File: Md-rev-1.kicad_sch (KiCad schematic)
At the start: 24 parts, among them CN1 JSTPH, J1 USB_C_Receptacle_USB2.0, J2 AudioJack4_SwitchTR1, U1 MCP73831-2-OT, U2 MAX9814

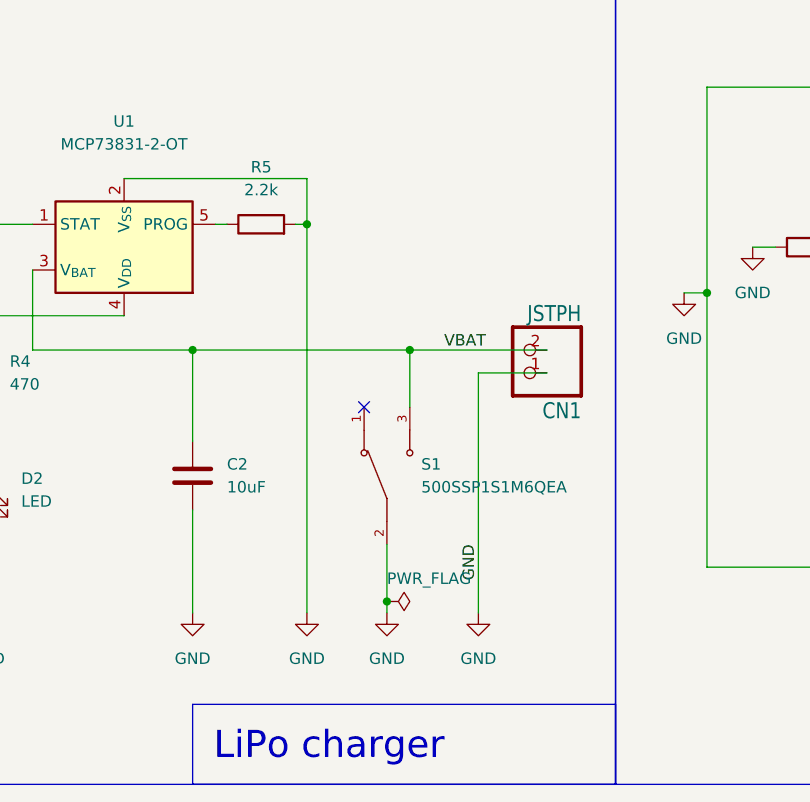
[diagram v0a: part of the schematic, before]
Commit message: Updated the schematic & PCB
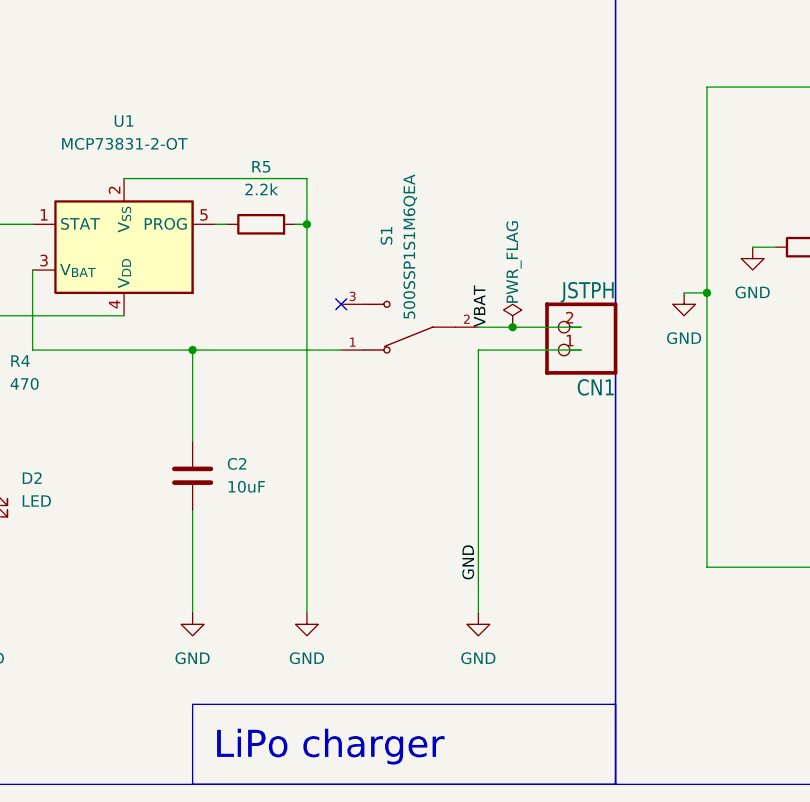
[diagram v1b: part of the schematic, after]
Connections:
- net GND: no longer S1.2
- net VBAT: now also S1.2; no longer C2.1, S1.3, U1.3 (V_{BAT})
- net at S1.1: now also C2.1, U1.3 (V_{BAT})
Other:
- moved on the sheet: CN1, S1
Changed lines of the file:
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@@
   (junction (at 180.34 118.11) (diameter 0) (color 0 0 0 0)
   )
-  (junction (at 144.78 152.4) (diameter 0) (color 0 0 0 0)
+  (junction (at 158.75 121.92) (diameter 0) (color 0 0 0 0)
   )
   (junction (at 123.19 124.46) (diameter 0) (color 0 0 0 0)
@@
   (junction (at 34.29 148.59) (diameter 0) (color 0 0 0 0)
   )
-  (junction (at 147.32 124.46) (diameter 0) (color 0 0 0 0)
-  )
   (junction (at 92.71 120.65) (diameter 0) (color 0 0 0 0)
   )
@@
   )
   (no_connect (at 345.44 124.46))
-  (no_connect (at 142.24 130.81))
+  (no_connect (at 139.7 119.38))
   (no_connect (at 62.23 123.19))
   (no_connect (at 62.23 130.81))
@@
     (stroke (width 0) (type default))
   )
-  (wire (pts (xy 154.94 127) (xy 154.94 153.67))
+  (wire (pts (xy 154.94 124.46) (xy 154.94 153.67))
     (stroke (width 0) (type default))
   )
@@
     (stroke (width 0) (type default))
   )
-  (wire (pts (xy 154.94 127) (xy 162.56 127))
+  (wire (pts (xy 154.94 124.46) (xy 166.37 124.46))
     (stroke (width 0) (type default))
   )
@@
     (stroke (width 0) (type default))
   )
+  (wire (pts (xy 154.94 121.92) (xy 158.75 121.92))
+    (stroke (width 0) (type default))
+  )
   (wire (pts (xy 57.15 123.19) (xy 62.23 123.19))
     (stroke (width 0) (type default))
@@
     (stroke (width 0) (type default))
   )
-  (wire (pts (xy 144.78 146.05) (xy 144.78 152.4))
-    (stroke (width 0) (type default))
-  )
   (wire (pts (xy 105.41 124.46) (xy 123.19 124.46))
     (stroke (width 0) (type default))
@@
     (stroke (width 0) (type default))
   )
-  (wire (pts (xy 123.19 124.46) (xy 147.32 124.46))
-    (stroke (width 0) (type default))
-  )
   (wire (pts (xy 185.42 113.03) (xy 187.96 113.03))
     (stroke (width 0) (type default))
@@
     (stroke (width 0) (type default))
   )
-  (wire (pts (xy 144.78 152.4) (xy 144.78 153.67))
-    (stroke (width 0) (type default))
-  )
   (wire (pts (xy 285.75 120.65) (xy 297.18 120.65))
     (stroke (width 0) (type default))
@@
     (stroke (width 0) (type default))
   )
-  (wire (pts (xy 147.32 124.46) (xy 147.32 130.81))
-    (stroke (width 0) (type default))
-  )
   (wire (pts (xy 200.66 113.03) (xy 240.03 113.03))
     (stroke (width 0) (type default))
@@
     (stroke (width 0) (type default))
   )
-  (wire (pts (xy 147.32 124.46) (xy 162.56 124.46))
+  (wire (pts (xy 123.19 124.46) (xy 139.7 124.46))
     (stroke (width 0) (type default))
   )
@@
   )
   (wire (pts (xy 123.19 142.24) (xy 123.19 153.67))
+    (stroke (width 0) (type default))
+  )
+  (wire (pts (xy 158.75 121.92) (xy 166.37 121.92))
     (stroke (width 0) (type default))
   )
@@
     (effects (font (size 1.27 1.27)) (justify left bottom))
   )
-  (label "VBAT" (at 151.13 124.46 0) (fields_autoplaced)
+  (label "VBAT" (at 156.21 121.92 90) (fields_autoplaced)
     (effects (font (size 1.27 1.27)) (justify left bottom))
   )
@@
     )
   )
-  (symbol (lib_id "500SSP1S1M6QEA:500SSP1S1M6QEA") (at 144.78 138.43 90) (unit 1)
-    (in_bom yes) (on_board yes) (dnp no) (fields_autoplaced)
-    (property "Reference" "S1" (at 148.59 137.16 90)
-      (effects (font (size 1.27 1.27)) (justify right))
-    )
-    (property "Value" "500SSP1S1M6QEA" (at 148.59 139.7 90)
-      (effects (font (size 1.27 1.27)) (justify right))
-    )
-    (property "Footprint" "500SSP1S1M6QEA:SW_500SSP1S1M6QEA" (at 144.78 138.43 0)
-      (effects (font (size 1.27 1.27)) (justify bottom) hide)
-    )
-    (property "Datasheet" "" (at 144.78 138.43 0)
-      (effects (font (size 1.27 1.27)) hide)
-    )
-    (property "MF" "E-Switch" (at 144.78 138.43 0)
-      (effects (font (size 1.27 1.27)) (justify bottom) hide)
-    )
-    (property "Description" "\nSlide Switch, 500A Series, DPDT, ON-ON, 5A, 120VAC/28VDC, Silver, R/A PC Pin | E-Switch 500SSP1S1M6QEA\n" (at 144.78 138.43 0)
-      (effects (font (size 1.27 1.27)) (justify bottom) hide)
-    )
-    (property "Package" "None" (at 144.78 138.43 0)
-      (effects (font (size 1.27 1.27)) (justify bottom) hide)
-    )
-    (property "Price" "None" (at 144.78 138.43 0)
-      (effects (font (size 1.27 1.27)) (justify bottom) hide)
-    )
-    (property "Check_prices" "https://www.snapeda.com/parts/500SSP1S1M6QEA/E-Switch/view-part/?ref=eda" (at 144.78 138.43 0)
-      (effects (font (size 1.27 1.27)) (justify bottom) hide)
-    )
-    (property "SnapEDA_Link" "https://www.snapeda.com/parts/500SSP1S1M6QEA/E-Switch/view-part/?ref=snap" (at 144.78 138.43 0)
-      (effects (font (size 1.27 1.27)) (justify bottom) hide)
-    )
-    (property "MP" "500SSP1S1M6QEA" (at 144.78 138.43 0)
-      (effects (font (size 1.27 1.27)) (justify bottom) hide)
-    )
-    (property "Availability" "In Stock" (at 144.78 138.43 0)
-      (effects (font (size 1.27 1.27)) (justify bottom) hide)
-    )
-    (property "Purchase-URL" "https://www.snapeda.com/api/url_track_click_mouser/?unipart_id=488032&manufacturer=E-Switch&part_name=500SSP1S1M6QEA&search_term=spdt" (at 144.78 138.43 0)
+  (symbol (lib_id "500SSP1S1M6QEA:500SSP1S1M6QEA") (at 147.32 121.92 180) (unit 1)
+    (in_bom yes) (on_board yes) (dnp no)
+    (property "Reference" "S1" (at 144.78 111.76 90)
+      (effects (font (size 1.27 1.27)))
+    )
+    (property "Value" "500SSP1S1M6QEA" (at 147.32 113.03 90)
+      (effects (font (size 1.27 1.27)))
+    )
+    (property "Footprint" "500SSP1S1M6QEA:SW_500SSP1S1M6QEA" (at 147.32 121.92 0)
+      (effects (font (size 1.27 1.27)) (justify bottom) hide)
+    )
+    (property "Datasheet" "" (at 147.32 121.92 0)
+      (effects (font (size 1.27 1.27)) hide)
+    )
+    (property "MF" "E-Switch" (at 147.32 121.92 0)
+      (effects (font (size 1.27 1.27)) (justify bottom) hide)
+    )
+    (property "Description" "\nSlide Switch, 500A Series, DPDT, ON-ON, 5A, 120VAC/28VDC, Silver, R/A PC Pin | E-Switch 500SSP1S1M6QEA\n" (at 147.32 121.92 0)
+      (effects (font (size 1.27 1.27)) (justify bottom) hide)
+    )
+    (property "Package" "None" (at 147.32 121.92 0)
+      (effects (font (size 1.27 1.27)) (justify bottom) hide)
+    )
+    (property "Price" "None" (at 147.32 121.92 0)
+      (effects (font (size 1.27 1.27)) (justify bottom) hide)
+    )
+    (property "Check_prices" "https://www.snapeda.com/parts/500SSP1S1M6QEA/E-Switch/view-part/?ref=eda" (at 147.32 121.92 0)
+      (effects (font (size 1.27 1.27)) (justify bottom) hide)
+    )
+    (property "SnapEDA_Link" "https://www.snapeda.com/parts/500SSP1S1M6QEA/E-Switch/view-part/?ref=snap" (at 147.32 121.92 0)
+      (effects (font (size 1.27 1.27)) (justify bottom) hide)
+    )
+    (property "MP" "500SSP1S1M6QEA" (at 147.32 121.92 0)
+      (effects (font (size 1.27 1.27)) (justify bottom) hide)
+    )
+    (property "Availability" "In Stock" (at 147.32 121.92 0)
+      (effects (font (size 1.27 1.27)) (justify bottom) hide)
+    )
+    (property "Purchase-URL" "https://www.snapeda.com/api/url_track_click_mouser/?unipart_id=488032&manufacturer=E-Switch&part_name=500SSP1S1M6QEA&search_term=spdt" (at 147.32 121.92 0)
       (effects (font (size 1.27 1.27)) (justify bottom) hide)
     )
@@
     )
   )
-  (symbol (lib_id "power:PWR_FLAG") (at 144.78 152.4 270) (unit 1)
+  (symbol (lib_id "power:PWR_FLAG") (at 158.75 121.92 0) (unit 1)
     (in_bom yes) (on_board yes) (dnp no)
-    (property "Reference" "#FLG02" (at 146.685 152.4 0)
-      (effects (font (size 1.27 1.27)) hide)
-    )
-    (property "Value" "PWR_FLAG" (at 144.78 149.86 90)
+    (property "Reference" "#FLG02" (at 158.75 120.015 0)
+      (effects (font (size 1.27 1.27)) hide)
+    )
+    (property "Value" "PWR_FLAG" (at 158.75 119.38 90)
       (effects (font (size 1.27 1.27)) (justify left))
     )
-    (property "Footprint" "" (at 144.78 152.4 0)
-      (effects (font (size 1.27 1.27)) hide)
-    )
-    (property "Datasheet" "~" (at 144.78 152.4 0)
+    (property "Footprint" "" (at 158.75 121.92 0)
+      (effects (font (size 1.27 1.27)) hide)
+    )
+    (property "Datasheet" "~" (at 158.75 121.92 0)
       (effects (font (size 1.27 1.27)) hide)
     )
@@
     )
   )
-  (symbol (lib_id "power:GND") (at 144.78 153.67 0) (unit 1)
-    (in_bom yes) (on_board yes) (dnp no) (fields_autoplaced)
-    (property "Reference" "#PWR08" (at 144.78 160.02 0)
-      (effects (font (size 1.27 1.27)) hide)
-    )
-    (property "Value" "GND" (at 144.78 158.75 0)
-      (effects (font (size 1.27 1.27)))
-    )
-    (property "Footprint" "" (at 144.78 153.67 0)
-      (effects (font (size 1.27 1.27)) hide)
-    )
-    (property "Datasheet" "" (at 144.78 153.67 0)
-      (effects (font (size 1.27 1.27)) hide)
-    )
-    (pin "1")
-    (instances
-      (project "Md-rev-1"
-        (path "/34e1f0a2-75b5-46dc-b967-b4433c15cc45"
-          (reference "#PWR08") (unit 1)
-        )
-      )
-    )
-  )
   (symbol (lib_id "Device:C") (at 123.19 138.43 0) (unit 1)
     (in_bom yes) (on_board yes) (dnp no)
@@
     )
   )
-  (symbol (lib_id "Adafruit USB C microlipo charger-eagle-import:JST_2PIN") (at 160.02 124.46 180) (unit 1)
+  (symbol (lib_id "Adafruit USB C microlipo charger-eagle-import:JST_2PIN") (at 163.83 121.92 180) (unit 1)
     (in_bom yes) (on_board yes) (dnp no)
-    (property "Reference" "CN1" (at 166.37 130.175 0)
+    (property "Reference" "CN1" (at 170.18 127.635 0)
       (effects (font (size 1.778 1.5113)) (justify left bottom))
     )
-    (property "Value" "JSTPH" (at 166.37 119.38 0)
+    (property "Value" "JSTPH" (at 170.18 116.84 0)
       (effects (font (size 1.778 1.5113)) (justify left bottom))
     )
-    (property "Footprint" "Connector_JST:JST_PH_S2B-PH-K_1x02_P2.00mm_Horizontal" (at 160.02 124.46 0)
-      (effects (font (size 1.27 1.27)) hide)
-    )
-    (property "Datasheet" "" (at 160.02 124.46 0)
-      (effects (font (size 1.27 1.27)) hide)
-    )
+    (property "Footprint" "Connector_JST:JST_PH_S2B-PH-K_1x02_P2.00mm_Horizontal" (at 163.83 121.92 0)
+      (effects (font (size 1.27 1.27)) hide)
+    )
+    (property "Datasheet" "" (at 163.83 121.92 0)
+      (effects (font (size 1.27 1.27)) hide)
+    )

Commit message: Updated the footprint files
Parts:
- MK1: footprint Buzzer_Beeper:MagneticBuzzer_Kingstate_KCG0601 -> Buzzer_Beeper:MagneticBuzzer_Kobitone_254-EMB73-RO
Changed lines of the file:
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@@
       (effects (font (size 1.27 1.27)))
     )
-    (property "Footprint" "Buzzer_Beeper:MagneticBuzzer_Kingstate_KCG0601" (at 207.01 128.27 90)
+    (property "Footprint" "Buzzer_Beeper:MagneticBuzzer_Kobitone_254-EMB73-RO" (at 207.01 128.27 90)
       (effects (font (size 1.27 1.27)) hide)
     )
